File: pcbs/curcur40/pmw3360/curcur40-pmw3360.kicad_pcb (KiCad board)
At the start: 2 copper layers, 21.8 x 26.5 mm, 20 parts, among them J1 Conn_01x08, U1 PMW3360DM-T2QU, U2 TLV74318PDBVR

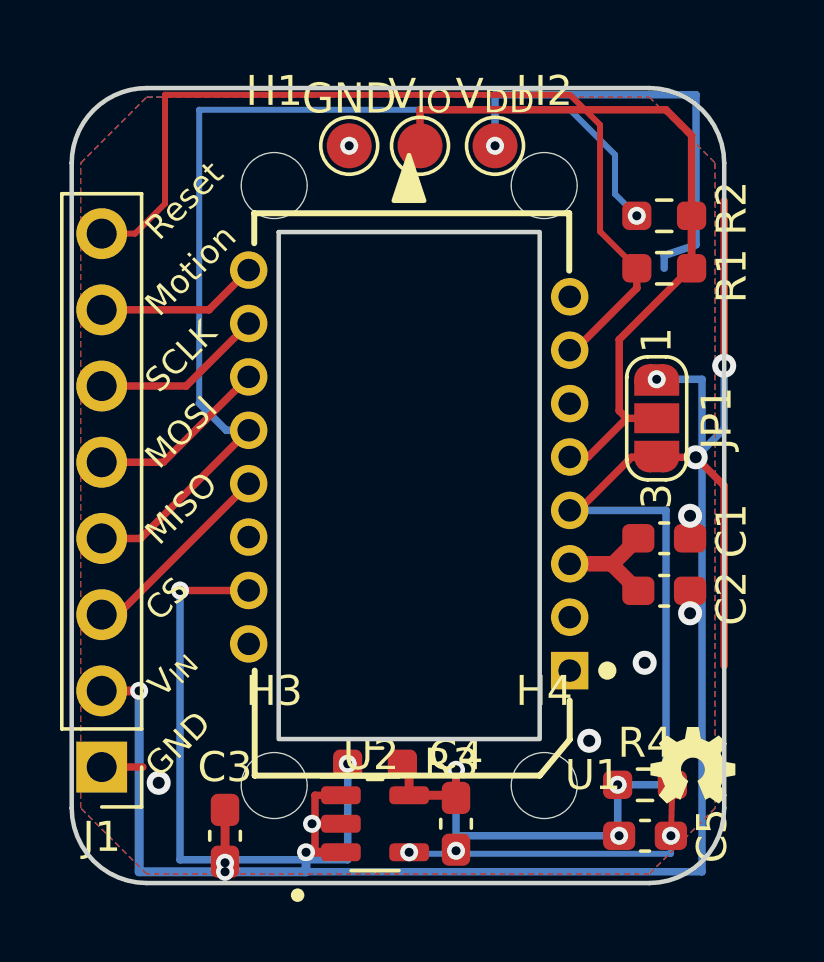
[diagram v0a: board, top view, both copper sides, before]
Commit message: fix error
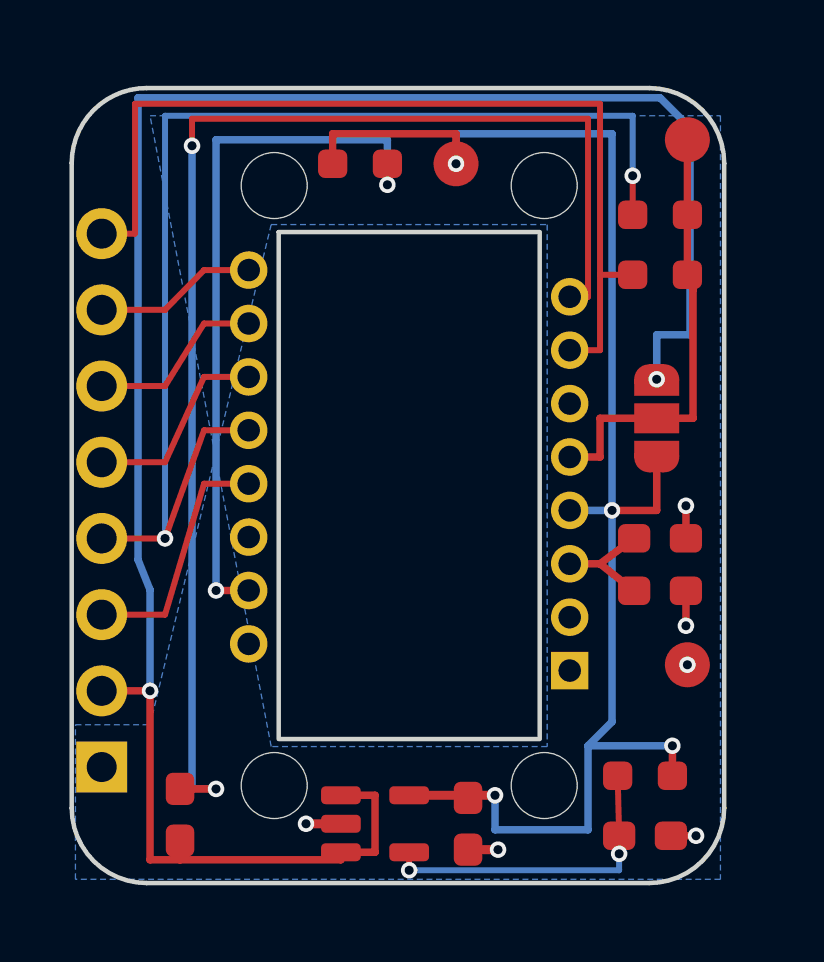
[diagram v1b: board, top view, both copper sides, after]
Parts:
- moved TP3 20.6 mm to (154.9, 98.5)
- moved R3 20.0 mm to (144.0, 81.8), turned to 0 degrees
- moved TP1 8.91 mm to (154.9, 81.0)
- moved C3 1.66 mm to (138.0, 103.5), turned to 90 degrees
- moved TP2 1.43 mm to (147.2, 81.8)
- moved C4 0.40 mm to (147.6, 103.8)
- moved R4 0.30 mm to (153.5, 102.2), turned to 180 degrees
- moved R1 0.26 mm to (154.0, 85.5)
- moved R2 0.14 mm to (154.0, 83.5)
- moved C1 0.14 mm to (154.0, 94.3)
- moved C2 0.14 mm to (154.0, 96.0)
- turned C5 to 0 degrees
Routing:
- net GND: track 2.34 -> 49.3 mm, vias 10 -> 8
- net V_{IN}: track 51.5 -> 66.8 mm, vias 4 -> 2
- net V_{IO}: track 26.4 -> 14.7 mm
- net VDD: track 63.2 -> 51.5 mm, vias 5 -> 4
- net /MISO: track 35.0 -> 40.4 mm, vias 1 -> 2
- net Net-(U1-LED_P): track 20.1 -> 24.0 mm
- net /CS: track 6.71 -> 8.15 mm
- net Net-(U1-VDDPIX): track 5.30 -> 3.88 mm
- net /RESET: track 30.1 -> 31.3 mm
- net /MOSI: track 6.08 -> 6.73 mm
- removed copper zone on F.Cu, net GND
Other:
- board text removed: "${TITLE} Rev ${REVISION}"
- board text removed: "CS"
- board text removed: "GND"
- board text removed: "JP1: [1-2 3]V_{IO}=V_{IN} [1 2-3]V_{IO}=V_{DD}"
- board text removed: "MISO"
- board text removed: "MOSI"
- board text removed: "Motion"
- board text removed: "Reset"
- board text removed: "SCLK"
- board text removed: "V_{IN}"
